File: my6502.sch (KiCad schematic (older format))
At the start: 69 parts, among them J1 Conn_01x08, J2 Conn_01x08, J3 Conn_01x08, J4 USB_B_Micro, SW1 Switch, SW2 SW_MEC_5G, SW3 SW_Push_DPDT, SW4 SW_Push, SW5 SW_Push, SW6 SW_Push, SW7 SW_Push, SW8 SW_Push, SW9 SW_Push, U1 74HC00, U12 74HC00, U17 74HC00, U18 LM555xN, U2 LM555xN, U3 W65C02S, U4 LM555xN, U5 28C256, U6 65C22, U7 CY62256-70PC, U8 HD44780, U9 74HC00, X1 CXO_DIP14

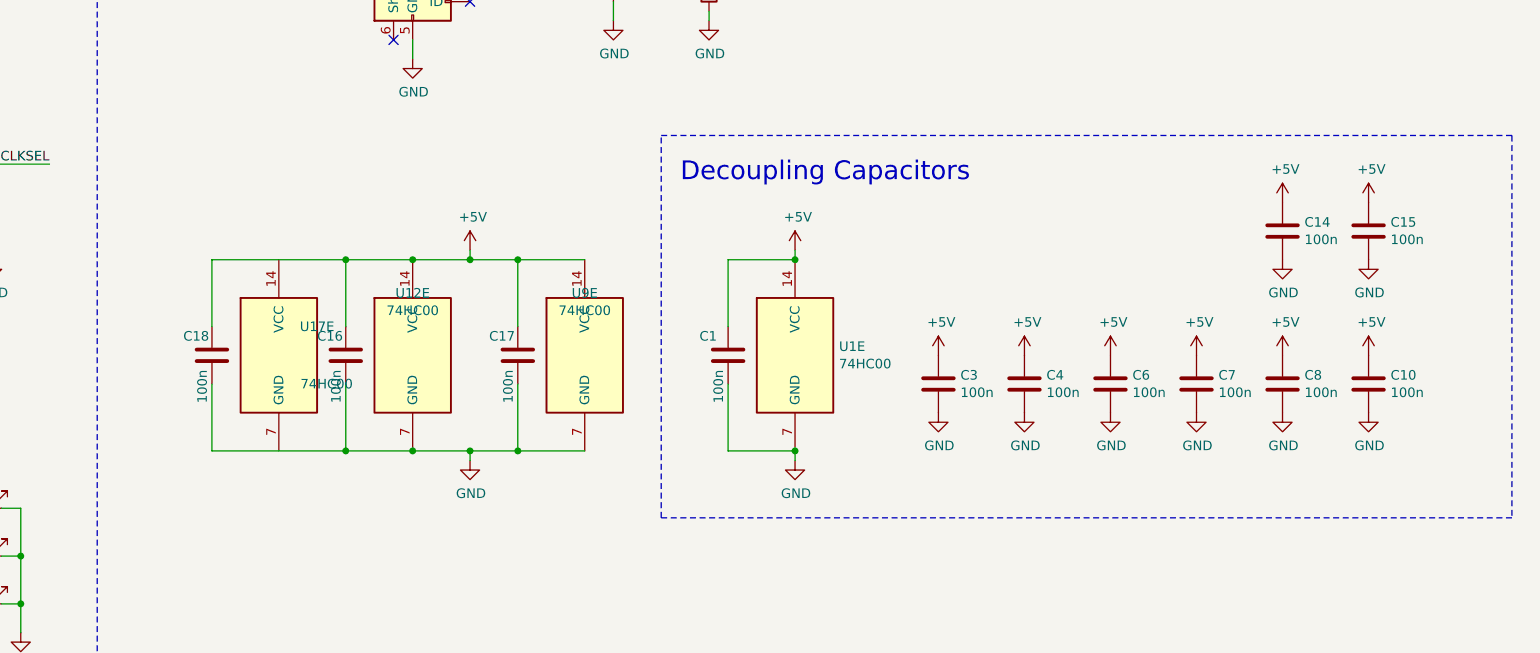
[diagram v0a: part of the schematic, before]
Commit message: Mostly minor adjustments
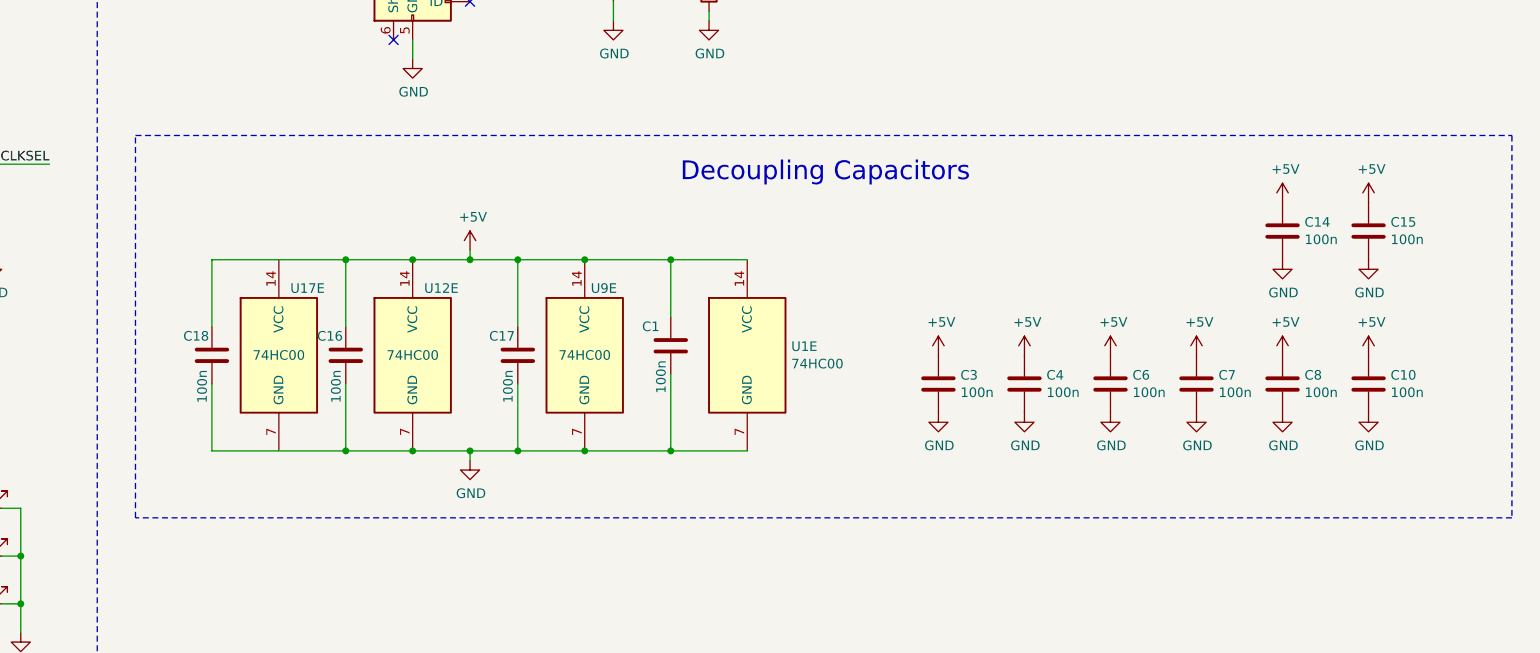
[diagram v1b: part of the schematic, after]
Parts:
- RV2, RV3: footprint Resistor_THT:R_Axial_DIN0207_L6.3mm_D2.5mm_P7.62mm_Horizontal -> Potentiometer_THT:Potentiometer_Piher_PT-6-V_Vertical
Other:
- moved on the sheet: C1, U1E
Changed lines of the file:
@@
 L 74xx:74HC00 U1
 U 5 1 6018728D
-P 12150 8950
-F 0 "U1" H 12380 8996 50  0000 L CNN
-F 1 "74HC00" H 12380 8905 50  0000 L CNN
-F 2 "Package_DIP:DIP-14_W7.62mm_LongPads" H 12150 8950 50  0001 C CNN
-F 3 "http://www.ti.com/lit/gpn/sn74hc00" H 12150 8950 50  0001 C CNN
-	5    12150 8950
+P 11900 8950
+F 0 "U1" H 12130 8996 50  0000 L CNN
+F 1 "74HC00" H 12130 8905 50  0000 L CNN
+F 2 "Package_DIP:DIP-14_W7.62mm_LongPads" H 11900 8950 50  0001 C CNN
+F 3 "http://www.ti.com/lit/gpn/sn74hc00" H 11900 8950 50  0001 C CNN
+	5    11900 8950
 	1    0    0    -1
 $EndComp
@@
 L Device:C C1
 U 1 1 6018D610
-P 11800 8950
-F 0 "C1" H 11650 9050 50  0000 L CNN
-F 1 "100n" V 11750 8700 50  0000 L CNN
-F 2 "Capacitor_THT:C_Disc_D5.1mm_W3.2mm_P5.00mm" H 11838 8800 50  0001 C CNN
-F 3 "~" H 11800 8950 50  0001 C CNN
-	1    11800 8950
+P 11500 8900
+F 0 "C1" H 11350 9000 50  0000 L CNN
+F 1 "100n" V 11450 8650 50  0000 L CNN
+F 2 "Capacitor_THT:C_Disc_D5.1mm_W3.2mm_P5.00mm" H 11538 8750 50  0001 C CNN
+F 3 "~" H 11500 8900 50  0001 C CNN
+	1    11500 8900
 	1    0    0    -1
 $EndComp
 Wire Wire Line
-	11800 8800 11800 8450
+	11500 8450 11900 8450
 Wire Wire Line
-	11800 8450 12150 8450
+	11500 9050 11500 9450
 Wire Wire Line
-	11800 9100 11800 9450
-Wire Wire Line
-	11800 9450 12150 9450
-$Comp
-L power:+5V #PWR0113
-U 1 1 601B7EDC
-P 12150 8400
-F 0 "#PWR0113" H 12150 8250 50  0001 C CNN
-F 1 "+5V" H 12165 8573 50  0000 C CNN
-F 2 "" H 12150 8400 50  0001 C CNN
-F 3 "" H 12150 8400 50  0001 C CNN
-	1    12150 8400
-	1    0    0    -1
-$EndComp
-Wire Wire Line
-	12150 8400 12150 8450
-$Comp
-L power:GND #PWR0114
-U 1 1 601BA2BC
-P 12150 9500
-F 0 "#PWR0114" H 12150 9250 50  0001 C CNN
-F 1 "GND" H 12155 9327 50  0000 C CNN
-F 2 "" H 12150 9500 50  0001 C CNN
-F 3 "" H 12150 9500 50  0001 C CNN
-	1    12150 9500
-	1    0    0    -1
-$EndComp
-Wire Wire Line
-	12150 9500 12150 9450
-Connection ~ 12150 9450
+	11500 9450 11900 9450
 $Comp
 L power:+5V #PWR0115
@@
 	1    0    0    -1
 $EndComp
-Connection ~ 12150 8450
 Wire Wire Line
 	2800 7200 2800 7250
@@
 Astable oscillator
 Wire Notes Line
-	11450 9800 11450 7800
+	8700 9800 8700 7800
 Wire Notes Line
-	11450 7800 15900 7800
+	8700 7800 15900 7800
 Wire Notes Line
 	15900 7800 15900 9800
 Wire Notes Line
-	15900 9800 11450 9800
+	15900 9800 8700 9800
 Text Notes 11550 8050 0    98   ~ 0
 Decoupling Capacitors
@@
 F 0 "RV2" H 12000 1600 50  0000 R CNN
 F 1 "10k?" H 12000 1500 50  0000 R CNN
-F 2 "Resistor_THT:R_Axial_DIN0207_L6.3mm_D2.5mm_P7.62mm_Horizontal" H 12100 1550 50  0001 C CNN
+F 2 "Potentiometer_THT:Potentiometer_Piher_PT-6-V_Vertical" H 12100 1550 50  0001 C CNN
 F 3 "~" H 12100 1550 50  0001 C CNN
 	1    12100 1550
@@
 F 0 "RV3" H 12150 2050 50  0000 R CNN
 F 1 "10k?" H 12150 1950 50  0000 R CNN
-F 2 "Resistor_THT:R_Axial_DIN0207_L6.3mm_D2.5mm_P7.62mm_Horizontal" H 12250 2000 50  0001 C CNN
+F 2 "Potentiometer_THT:Potentiometer_Piher_PT-6-V_Vertical" H 12250 2000 50  0001 C CNN
 F 3 "~" H 12250 2000 50  0001 C CNN
 	1    12250 2000
@@
 U 5 1 60C17C42
 P 11050 8950
-F 0 "U9" H 11050 9275 50  0000 C CNN
-F 1 "74HC00" H 11050 9184 50  0000 C CNN
+F 0 "U9" H 11150 9300 50  0000 C CNN
+F 1 "74HC00" H 11050 8950 50  0000 C CNN
 F 2 "Package_DIP:DIP-14_W7.62mm_LongPads" H 11050 8950 50  0001 C CNN
 F 3 "http://www.ti.com/lit/gpn/sn74hc00" H 11050 8950 50  0001 C CNN
@@
 U 5 1 60C78F3C
 P 10150 8950
-F 0 "U12" H 10150 9275 50  0000 C CNN
-F 1 "74HC00" H 10150 9184 50  0000 C CNN
+F 0 "U12" H 10300 9300 50  0000 C CNN
+F 1 "74HC00" H 10150 8950 50  0000 C CNN
 F 2 "Package_DIP:DIP-14_W7.62mm_LongPads" H 10150 8950 50  0001 C CNN
 F 3 "http://www.ti.com/lit/gpn/sn74hc00" H 10150 8950 50  0001 C CNN
@@
 U 5 1 60E661A5
 P 9450 8950
-F 0 "U17" H 9650 9100 50  0000 C CNN
-F 1 "74HC00" H 9700 8800 50  0000 C CNN
+F 0 "U17" H 9600 9300 50  0000 C CNN
+F 1 "74HC00" H 9450 8950 50  0000 C CNN
 F 2 "Package_DIP:DIP-14_W7.62mm_LongPads" H 9450 8950 50  0001 C CNN
 F 3 "http://www.ti.com/lit/gpn/sn74hc00" H 9450 8950 50  0001 C CNN
@@
 Wire Wire Line
 	11700 7150 11700 7200
+Text Notes -2500 600  0    50   ~ 0
+TODO:\n- Mounting holes\n- Check if any more 6502 pins\n    should be accessible (RDY? NMI?)\n- Validate all components! Not the least the USB conn.\n- Place all decoupler caps close to their IC's\n- Fancy silkscreen!\n- Is HLT connected anywhere?
+Wire Wire Line
+	11500 8750 11500 8450
+Wire Wire Line
+	11050 8450 11500 8450
+Connection ~ 11050 8450
+Connection ~ 11500 8450
+Wire Wire Line
+	11050 9450 11500 9450
+Connection ~ 11050 9450
+Connection ~ 11500 9450
 Wire Bus Line
-	9200 800  9200 2150
+	9650 900  9650 3550
 Wire Bus Line
-	6900 800  6900 2150
+	9200 800  9200 2150
 Wire Bus Line
-	7300 800  7300 2850
+	14000 900  14000 2550
 Wire Bus Line
 	4900 800  4900 2850
 Wire Bus Line
-	14000 900  14000 2550
-Wire Bus Line
-	9650 900  9650 3550
+	6900 800  6900 2150
 Wire Bus Line
 	4200 800  4200 4950
 Wire Bus Line
 	11700 800  11700 5500
-Text Notes -2500 600  0    50   ~ 0
-TODO:\n- Mounting holes\n- Check if any more 6502 pins\n    should be accessible (RDY? NMI?)\n- Validate all components! Not the least the USB conn.\n- Place all decoupler caps close to their IC's\n- Fancy silkscreen!\n- Is HLT connected anywhere?
+Wire Bus Line
+	7300 800  7300 2850
 $EndSCHEMATC
